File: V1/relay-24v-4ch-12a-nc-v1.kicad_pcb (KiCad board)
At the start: 2 copper layers, 68 x 67.8 mm, 24 parts, among them J1 DB141V-2.54-2P, J2 DB141V-2.54-4P, J3 DB142V-5.08-4P, J4 DB142V-5.08-4P, K1 Songle_SRD_1B, K2 Songle_SRD_1B, K3 Songle_SRD_1B, K4 Songle_SRD_1B

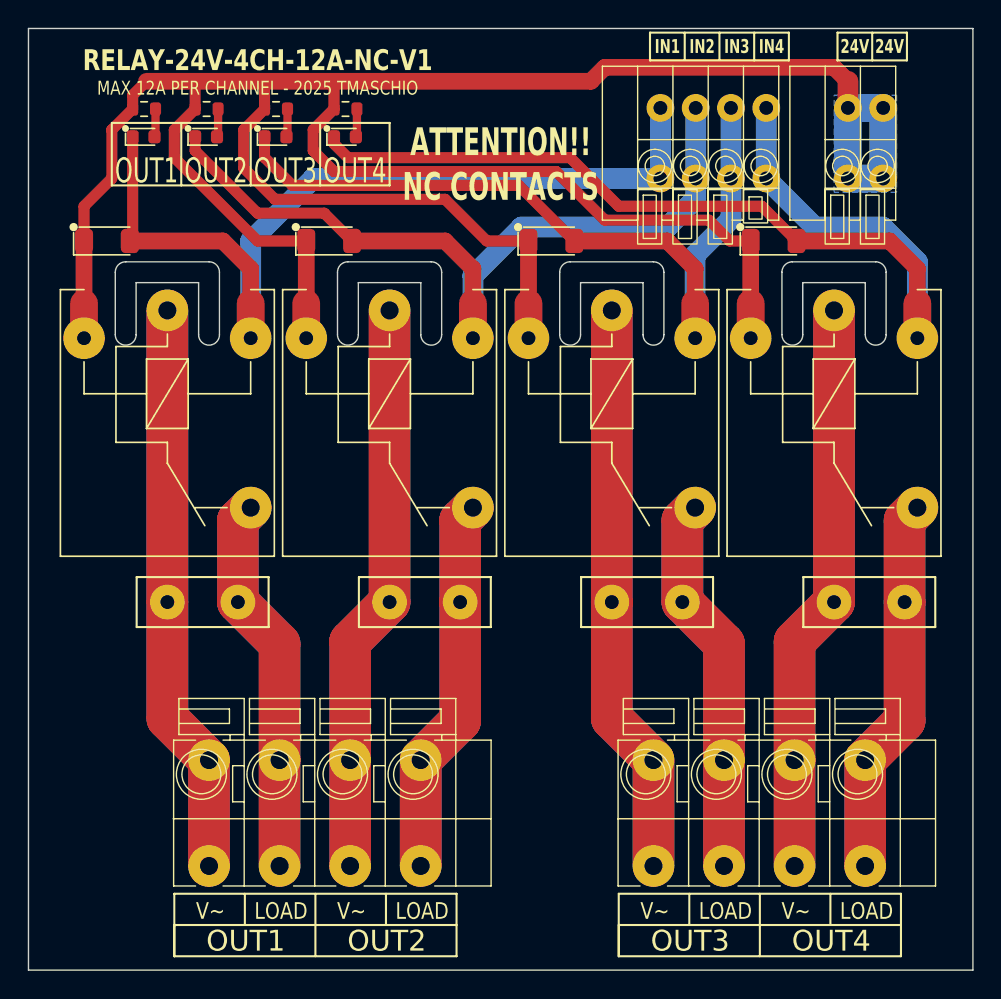
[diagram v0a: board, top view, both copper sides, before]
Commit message: Review before fabrication
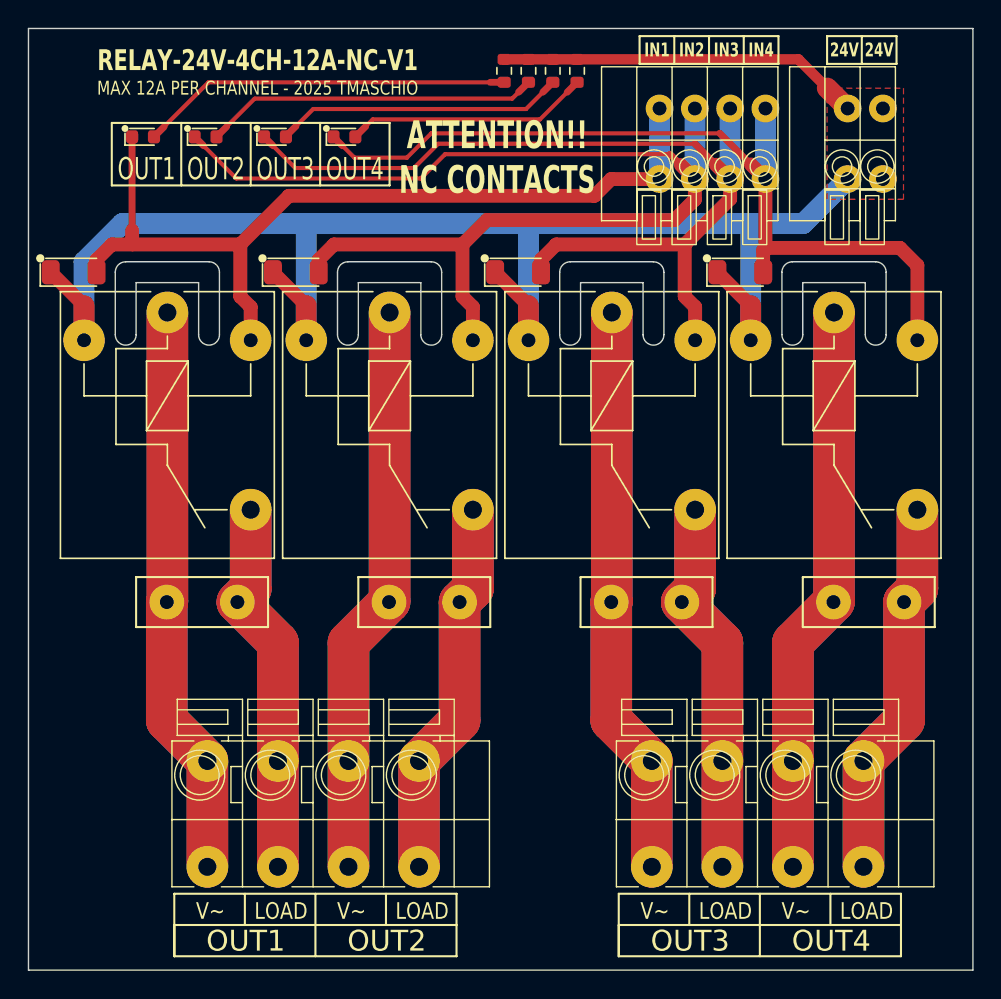
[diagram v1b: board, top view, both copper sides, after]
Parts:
- R1, R2, R3, R4: value 6k8/100mW -> 10k/100mW
- moved R1 26.1 mm to (159.2, 65.2), turned to -90 degrees
- moved R2 23.3 mm to (161.0, 65.2), turned to -90 degrees
- moved R3 20.1 mm to (162.8, 65.2), turned to -90 degrees
- moved R4 16.9 mm to (164.5, 65.2), turned to -90 degrees
- moved J3 8.39 mm to (145.5, 118.8)
- moved J4 8.39 mm to (177.5, 118.8)
- moved K1 7.25 mm to (135.0, 89.8)
- moved K2 7.25 mm to (151.0, 89.8)
- moved K3 7.25 mm to (167.0, 89.8)
- moved K4 7.25 mm to (183.0, 89.8)
- moved J2 4.65 mm to (174.2, 70.5)
- moved D2 3.29 mm to (128.2, 79.8)
- moved D4 3.29 mm to (144.2, 79.8)
- moved D6 3.29 mm to (160.2, 79.8)
- moved D8 3.29 mm to (176.2, 79.8)
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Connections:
- net Net-(D1-A) renamed /LED1
- net Net-(D1-K) renamed /IN1
- net Net-(D3-A) renamed /LED2
- net Net-(D3-K) renamed /IN2
- net Net-(D5-A) renamed /LED3
- net Net-(D5-K) renamed /IN3
- net Net-(D7-A) renamed /LED4
- net Net-(D7-K) renamed /IN4
- net Net-(J3-Pin_1) renamed /OUT1PW
- net Net-(J3-Pin_2) renamed /OUT1LD
- net Net-(J3-Pin_3) renamed /OUT2PW
- net Net-(J3-Pin_4) renamed /OUT2LD
- net Net-(J4-Pin_1) renamed /OUT3PW
- net Net-(J4-Pin_2) renamed /OUT3LD
- net Net-(J4-Pin_3) renamed /OUT4PW
- net Net-(J4-Pin_4) renamed /OUT4LD
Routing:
- net +24V: track 197.3 -> 138.1 mm
- net /LED1: track 2.03 -> 26.8 mm
- net /IN2: track 58.9 -> 82.3 mm
- net /LED2: track 2.03 -> 24.1 mm
- net /LED3: track 2.03 -> 20.9 mm
- net /LED4: track 2.03 -> 17.6 mm
- net /IN4: track 75.3 -> 62.5 mm
- net /IN3: track 58.5 -> 66.3 mm
- net /IN1: track 65.6 -> 63.9 mm
- added copper zone on F.Cu, net +24V
- removed copper zone on B.Cu, net +24V
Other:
- rule pad_to_mask_clearance: 0 -> 0.1
